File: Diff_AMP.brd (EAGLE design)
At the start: 25.7 x 20.6 mm, 23 parts, among them IC1 NCV8711ASN500T1G, IC3 MCP1501T-25E_RW, IC4 NCS21911SN2T1G, IC5 NCS21911SN2T1G

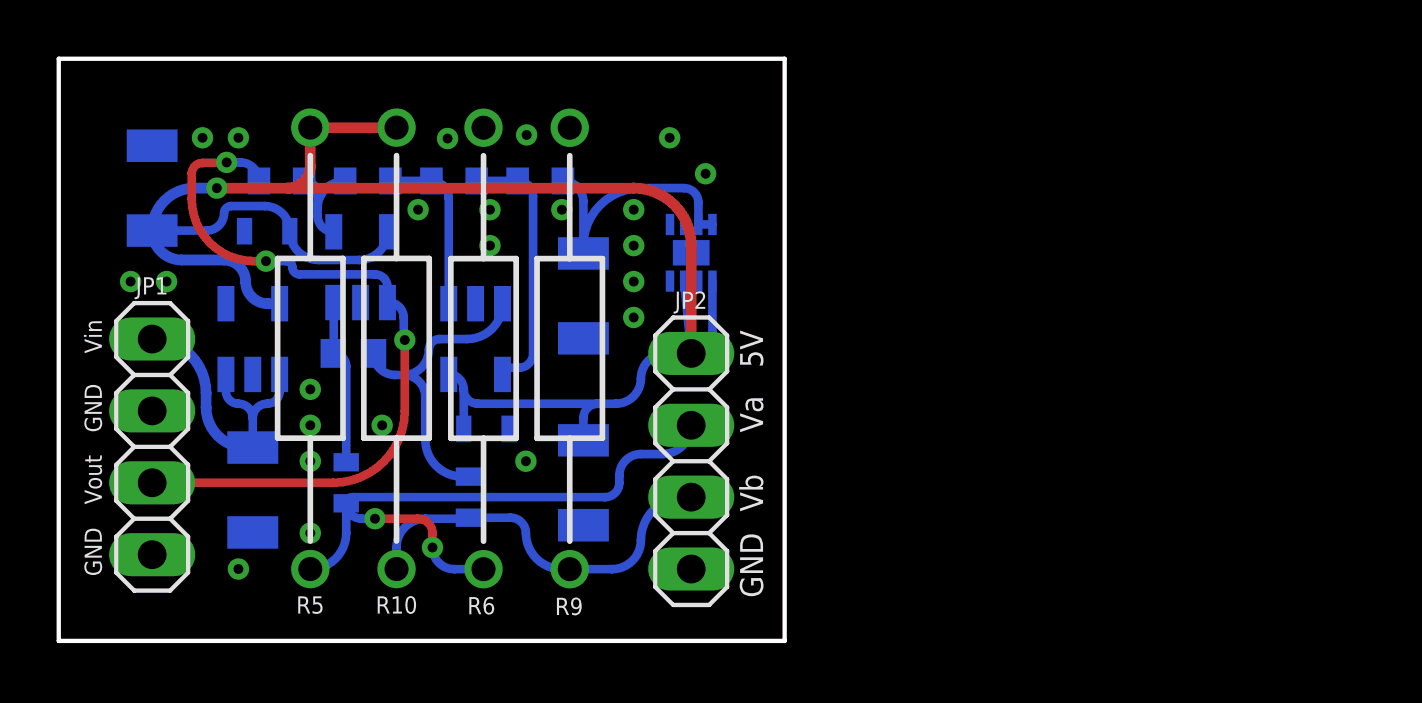
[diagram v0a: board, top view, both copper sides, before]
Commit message: revisions
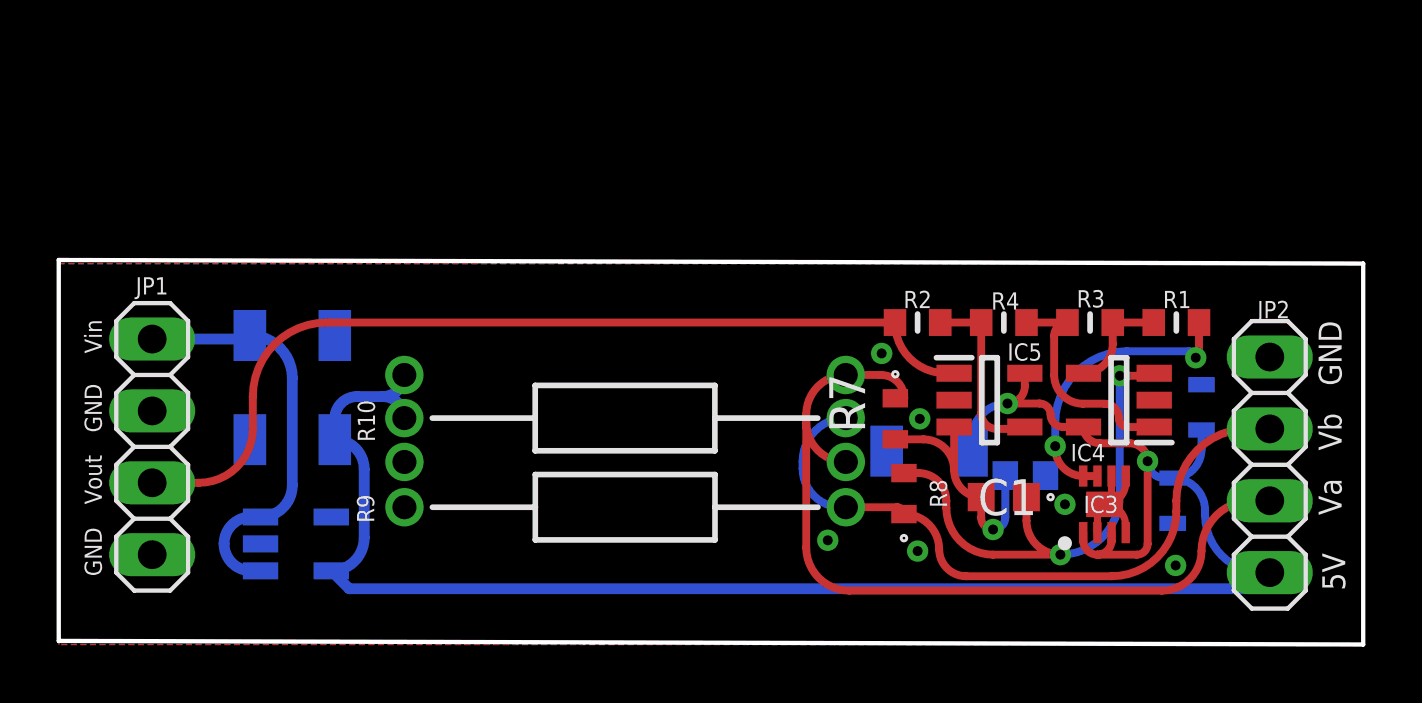
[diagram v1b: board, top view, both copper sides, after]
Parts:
- removed R11, R12: ERA-3VEB1911V, SamacSys_Parts:ERA3KV_(0603)
- added R7, R8: ERA-3VEB1911V, SamacSys_Parts:ERA3KV_(0603)
- C1: value C1206F105M5RACAUTO7210 -> C0603C184K3RACAUTO; device SamacSys_Parts:C1206 -> SamacSys_Parts:C0603
- moved C5 33.6 mm to (40.4, 8.26), turned to 270 degrees
- moved C4 24.4 mm to (39.4, 4.95), turned to 90 degrees
- moved C2 24.1 mm to (34.2, 5.84), turned to 180 degrees
- moved R2 23.0 mm to (30.4, 11.3), flipped to the top, turned to 180 degrees
- moved R4 23.0 mm to (33.4, 11.3), flipped to the top, turned to 180 degrees
- moved R1 23.0 mm to (39.5, 11.3), flipped to the top, turned to 180 degrees
- moved R3 23.0 mm to (36.4, 11.3), flipped to the top, turned to 180 degrees
- moved IC4 22.8 mm to (37.5, 8.51), flipped to the top, turned to 180 degrees
- moved IC5 22.7 mm to (32.9, 8.51), flipped to the top, turned to 0 degrees
- moved JP2 20.4 mm to (42.8, 6.22), turned to 90 degrees
- moved R5 20.1 mm to (27.8, 9.40), flipped to the bottom, turned to 0 degrees
- moved IC3 17.1 mm to (37.0, 4.83), flipped to the top
- moved R10 16.7 mm to (27.8, 7.87), turned to 180 degrees
- moved C1 16.5 mm to (33.4, 5.08), flipped to the top, turned to 180 degrees
- moved R9 14.6 mm to (12.2, 4.72), turned to 0 degrees
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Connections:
- net GND: now also C2.2; no longer C1.1
- net N$1: no longer C1.2
- net N$3: now also C1.1, R8.2; no longer C2.1, R11.2
- net N$9: now also C1.2, C2.1, R7.2; no longer C2.2, R12.2
- net VA: now also R7.1; no longer R12.1
- net VB: now also R8.1; no longer R11.1
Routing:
- net VB: track 13.4 -> 22.9 mm
- net VA: track 22.4 -> 29.7 mm, vias 2 -> 0
- net N$3: track 10.6 -> 17.8 mm, vias 0 -> 2
- net VOUT: track 26.6 -> 32.1 mm, vias 3 -> 0
- net N$2: track 9.16 -> 3.67 mm
- net 5V: track 63.4 -> 68.5 mm, vias 1 -> 2
- net GND: track 0.00 -> 4.83 mm, vias 23 -> 5
- net VIN: track 10.4 -> 14.4 mm
- net N$9: track 5.86 -> 8.80 mm, vias 0 -> 1
- net N$13: track 3.61 -> 6.46 mm
- net N$12: track 6.04 -> 7.79 mm
- net N$1: track 9.54 -> 10.2 mm, vias 0 -> 2
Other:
- board size 25.7 x 20.6 mm -> 46.1 x 13.6 mm
